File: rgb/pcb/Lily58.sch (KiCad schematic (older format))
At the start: 113 parts, among them J1 LED, J2 4PIN, P1 i2c_pin, P2 i2c_pin, P3 ICSP, P4 OLED, SW1 SW_PUSH, SW10 SW_PUSH, SW11 SW_PUSH, SW12 SW_PUSH, SW13 SW_PUSH, SW14 SW_PUSH, SW15 SW_PUSH, SW16 SW_PUSH, SW17 SW_PUSH, SW18 SW_PUSH, SW19 SW_PUSH, SW2 SW_PUSH, SW20 SW_PUSH, SW21 SW_PUSH, SW22 SW_PUSH, SW23 SW_PUSH, SW24 SW_PUSH, SW25 SW_PUSH, SW26 SW_PUSH, SW27 SW_PUSH, SW28 SW_PUSH, SW29 SW_PUSH, SW3 SW_PUSH, SW4 SW_PUSH, SW5 SW_PUSH, SW6 SW_PUSH, SW7 SW_PUSH, SW8 SW_PUSH, SW9 SW_PUSH, U1 ProMicro

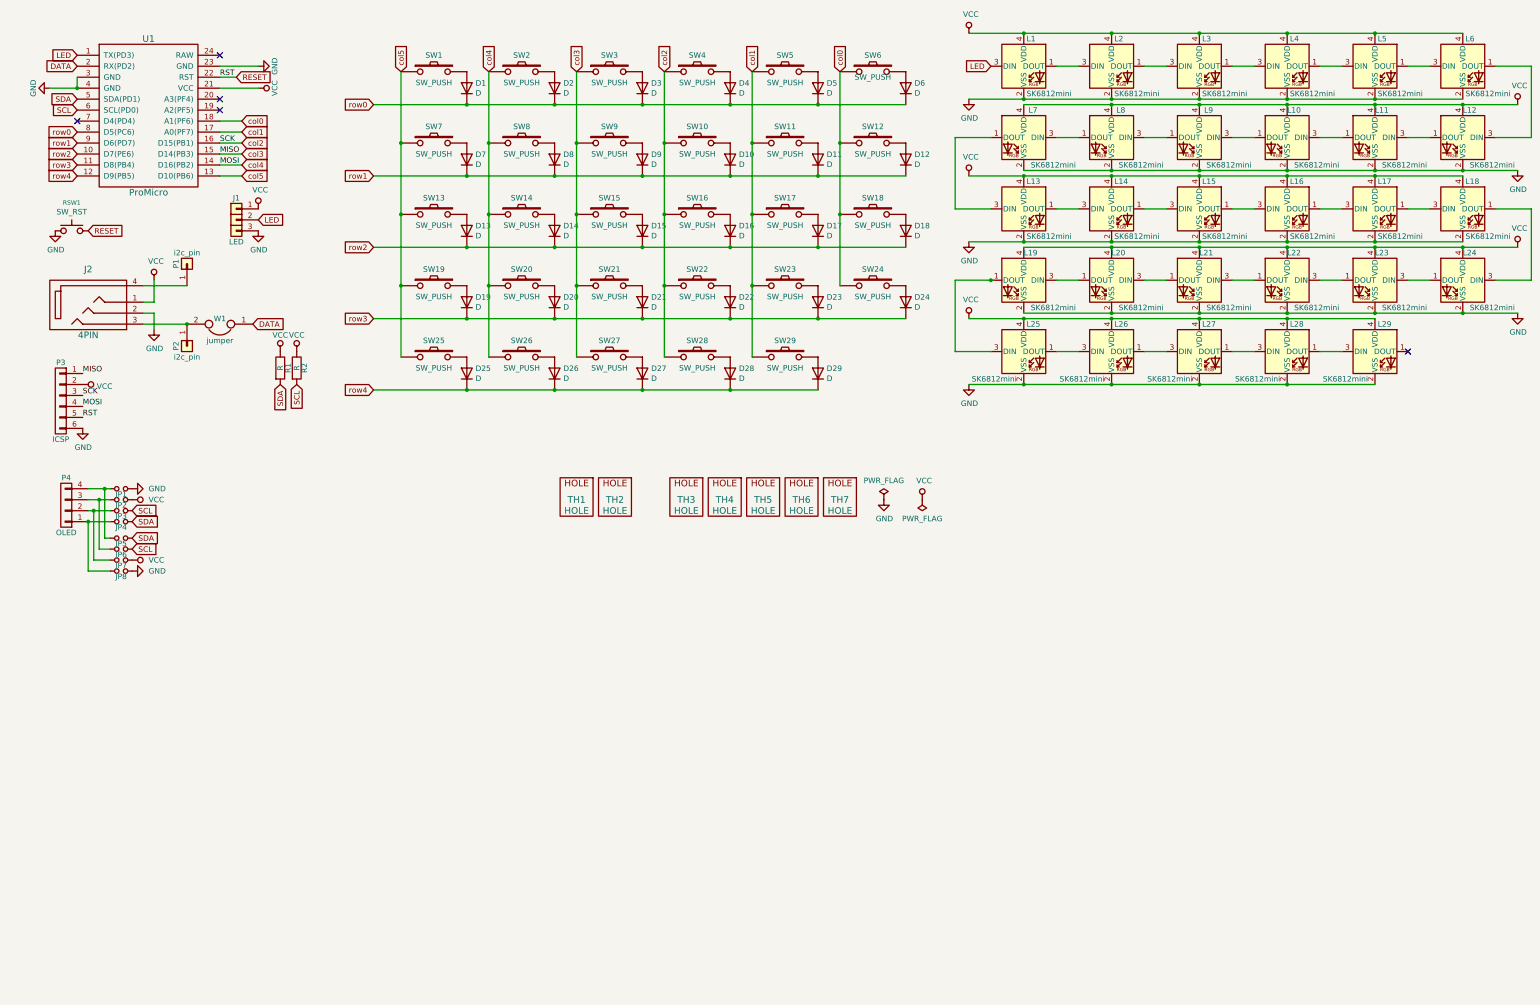
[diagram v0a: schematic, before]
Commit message: Add underglow
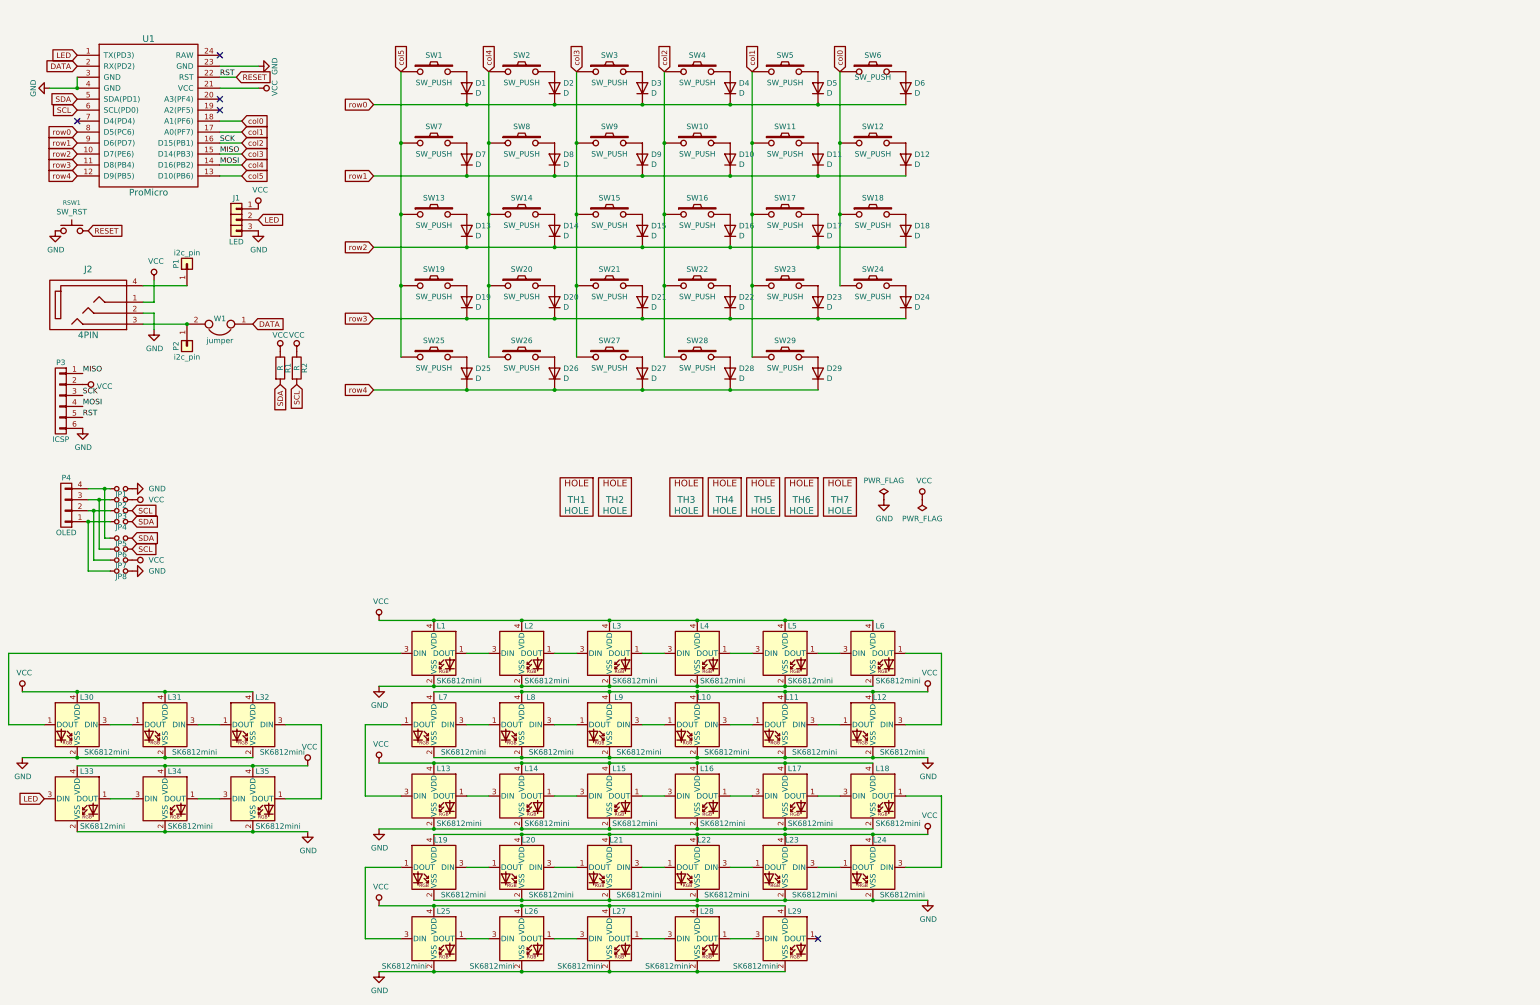
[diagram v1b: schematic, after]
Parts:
- added L30, L31, L32, L33, L34, L35: SK6812mini, Lily58-footprint:SK6812MINI_underglow_rev, symbol LED:SK6812MINI
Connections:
- net GND: now also L30.2 (VSS), L31.2 (VSS), L32.2 (VSS), L33.2 (VSS), L34.2 (VSS), L35.2 (VSS)
- net LED: now also L33.3 (DIN); no longer L1.3 (DIN)
- net VCC: now also L30.4 (VDD), L31.4 (VDD), L32.4 (VDD), L33.4 (VDD), L34.4 (VDD), L35.4 (VDD)
- new net: L1.3 (DIN), L30.1 (DOUT)
- new net: L30.3 (DIN), L31.1 (DOUT)
- new net: L31.3 (DIN), L32.1 (DOUT)
- new net: L32.3 (DIN), L35.1 (DOUT)
- new net: L34.1 (DOUT), L35.3 (DIN)
- new net: L33.1 (DOUT), L34.3 (DIN)
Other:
- moved on the sheet: L1, L10, L11, L12, L13, L14, L15, L16, L17, L18, L19, L2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
